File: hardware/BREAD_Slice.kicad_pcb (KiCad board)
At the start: 2 copper layers, 72.6 x 100 mm, 62 parts, among them J1 I2C_01x04, J2 Conn_01x10_Female, J3 Conn_01x02_Socket, J4 Conn_01x02_Socket, J5 Conn_01x02_Socket, J6 Conn_01x02_Socket, Q1 PSMN1R0-30YLC,115, Q2 PSMN1R0-30YLC,115, Q3 PSMN1R0-30YLC,115, Q4 PSMN1R0-30YLC,115, Q5 PSMN1R0-30YLC,115, Q6 PSMN1R0-30YLC,115, Q7 PSMN1R0-30YLC,115, Q8 PSMN1R0-30YLC,115

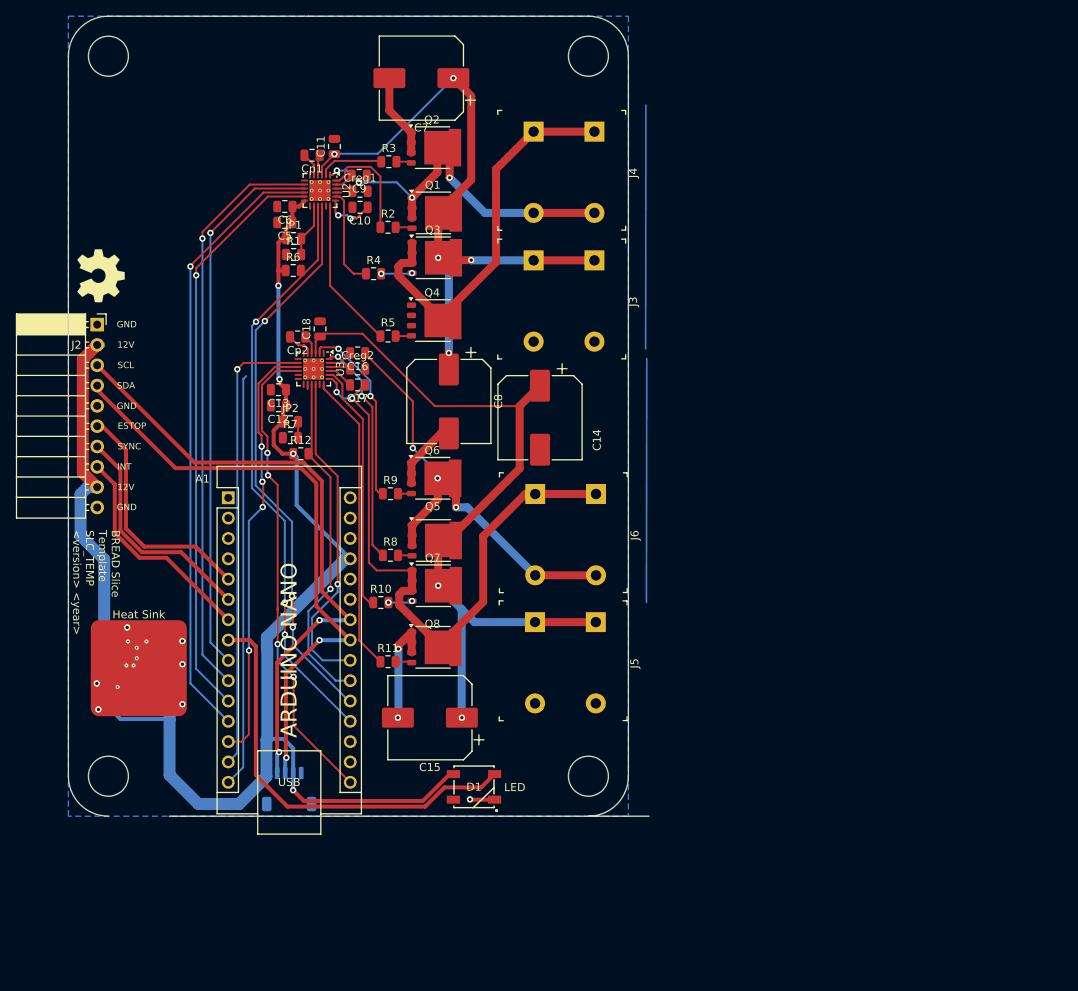
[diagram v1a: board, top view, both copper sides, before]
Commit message: removed old
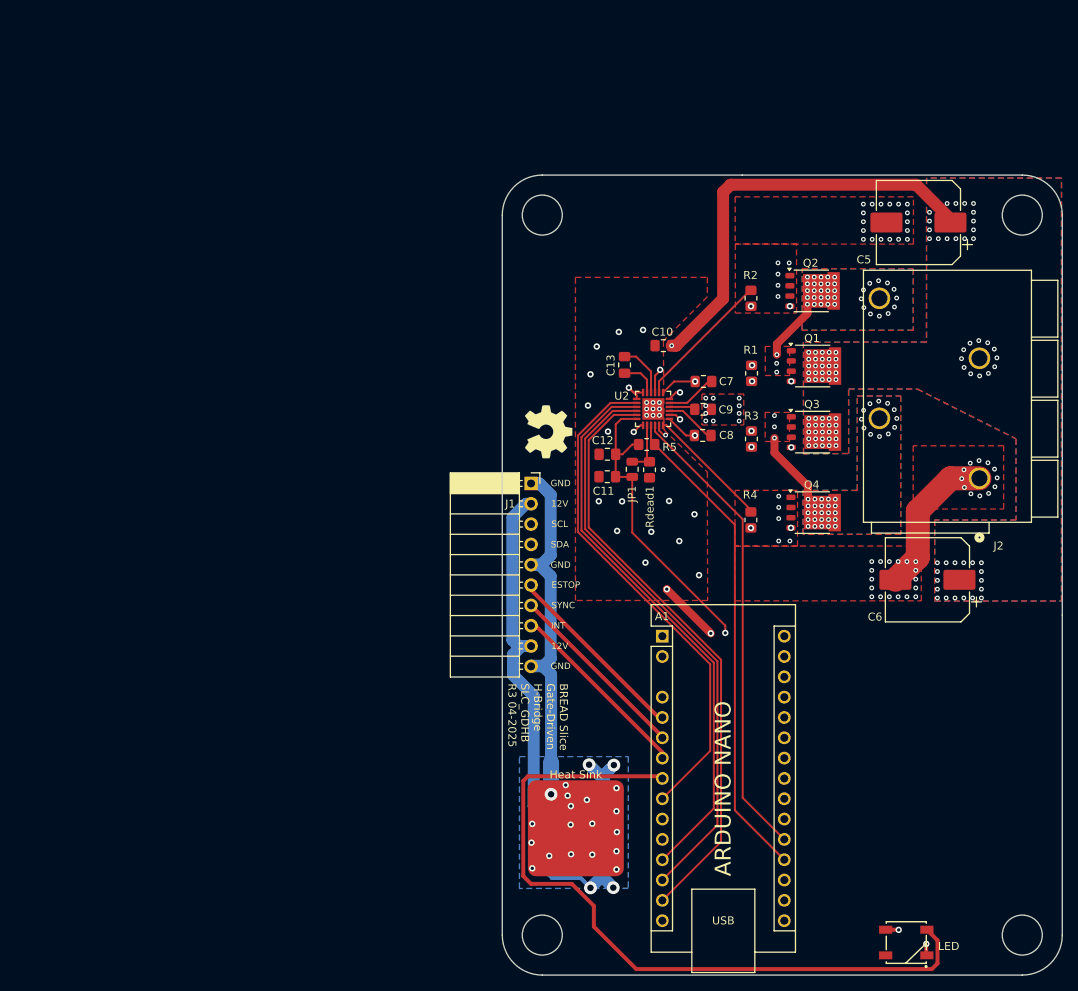
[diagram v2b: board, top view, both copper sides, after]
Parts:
- removed C14, C15: 50V 220uF, Capacitor_SMD:CP_Elec_10x10
- removed C16, C17: 1nF, Capacitor_SMD:C_0805_2012Metric
- removed C18: 50V 10uF, Capacitor_SMD:C_0805_2012Metric
- removed Cp1, Cp2: 16V 470nF, Capacitor_SMD:C_0805_2012Metric
- removed Creg1, Creg2: 16V 22uF, Capacitor_SMD:C_0805_2012Metric
- removed the J1 at (90.8, 121.6)
- removed J3, J4, J5, J6: Conn_01x02_Socket, Library:Term_Block_1x2_P10.16mm
- removed JP2: Jumper_2_Open, Capacitor_SMD:C_0805_2012Metric
- removed Q5, Q6, Q7, Q8: PSMN1R0-30YLC,115, Package_TO_SOT_SMD:LFPAK56
- removed R10, R11, R8, R9: 1K, Capacitor_SMD:C_0805_2012Metric
- removed R12, R6, R7: 10K, Capacitor_SMD:C_0805_2012Metric
- removed U3: ~, Package_DFN_QFN:HVQFN-24-1EP_4x4mm_P0.5mm_EP2.6x2.6mm_ThermalVias
- added J2: 2606-1104/010-000, kml-custom:CONN4_2606-1104&slash_010-000_WAG, F.Cu at (177.1, 82.8)
- added NT1: NetTie_2, NetTie:NetTie-2_SMD_Pad2.0mm, B.Cu at (123.6, 120.3)
- added Rdead1: 3k, Resistor_SMD:R_0805_2012Metric_Pad1.20x1.40mm_HandSolder, F.Cu at (135.9, 81.7)
- C1, C2, C3, C4: footprint Capacitor_SMD:C_1206_3216Metric -> Capacitor_SMD:C_1206_3216Metric_Pad1.33x1.80mm_HandSolder
- C10: value 1nF -> 50V 10uF; footprint Capacitor_SMD:C_0805_2012Metric -> Capacitor_SMD:C_0805_2012Metric_Pad1.18x1.45mm_HandSolder
- C11: value 50V 10uF -> 100nF; footprint Capacitor_SMD:C_0805_2012Metric -> Capacitor_SMD:C_0805_2012Metric_Pad1.18x1.45mm_HandSolder
- C12: footprint Capacitor_SMD:C_0805_2012Metric -> Capacitor_SMD:C_0805_2012Metric_Pad1.18x1.45mm_HandSolder
- C13: value 100nF -> 16V 470nF; footprint Capacitor_SMD:C_0805_2012Metric -> Capacitor_SMD:C_0805_2012Metric_Pad1.18x1.45mm_HandSolder
- C5: value 10uF -> 50V 220uF; footprint Capacitor_SMD:C_0805_2012Metric -> Capacitor_SMD:CP_Elec_10x10
- C6: value 100nF -> 50V 220uF; footprint Capacitor_SMD:C_0805_2012Metric -> Capacitor_SMD:CP_Elec_10x10
- C7, C8: value 50V 220uF -> 1nF; footprint Capacitor_SMD:CP_Elec_10x10 -> Capacitor_SMD:C_0805_2012Metric_Pad1.18x1.45mm_HandSolder
- C9: value 1nF -> 16V 22uF; footprint Capacitor_SMD:C_0805_2012Metric -> Capacitor_SMD:C_0805_2012Metric_Pad1.18x1.45mm_HandSolder
- HS1: footprint KML-Custom:Thermal Pad -> kml-custom:Thermal Pad
- R1: value 10K -> 1K; footprint Capacitor_SMD:C_0805_2012Metric -> Resistor_SMD:R_0805_2012Metric_Pad1.20x1.40mm_HandSolder
- R2, R3, R4: footprint Capacitor_SMD:C_0805_2012Metric -> Resistor_SMD:R_0805_2012Metric_Pad1.20x1.40mm_HandSolder
- R5: value 1K -> 10K; footprint Capacitor_SMD:C_0805_2012Metric -> Resistor_SMD:R_0805_2012Metric_Pad1.20x1.40mm_HandSolder
- U1: value ~ -> AP63205
- U2: value ~ -> A4957SESTR-T; footprint Package_DFN_QFN:HVQFN-24-1EP_4x4mm_P0.5mm_EP2.6x2.6mm_ThermalVias -> kml-custom:QFN-24_ALM
- moved C6 92.9 mm to (170.6, 95.5)
- moved C5 79.2 mm to (169.5, 50.8)
- moved Logo1 59.3 mm to (123.3, 77.0)
- moved R1 59.1 mm to (148.6, 69.7), turned to -90 degrees
- moved HS1 58.2 mm to (126.7, 126.5)
- moved C1 58.0 mm to (123.7, 124.6)
- moved C2 57.8 mm to (126.0, 131.3)
- moved H1 57.8 mm to (122.5, 49.9)
- moved H2 57.8 mm to (122.5, 139.9)
- moved J1 57.8 mm to (121.1, 83.4)
- moved U1 57.8 mm to (123.6, 127.8)
- moved C3 57.8 mm to (128.7, 124.5)
- moved H3 57.8 mm to (182.5, 49.9)
- moved H4 57.8 mm to (182.5, 139.9)
- moved L1 57.8 mm to (128.7, 127.8)
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- renumbered J2 to J1
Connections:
- net /E_STOP renamed /ESTOP
- A1 pad 10: /BLO1 -> unconnected-(A1-D7-Pad10)
- A1 pad 11: /AHI1 -> unconnected-(A1-D8-Pad11)
- A1 pad 12: /ALO1 -> /BHI1
- A1 pad 13: /BHI2 -> /ALO1
- A1 pad 14: /BLO2 -> /ALI1
- A1 pad 15: /AHI2 -> unconnected-(A1-D12-Pad15)
- A1 pad 16: /ALO2 -> unconnected-(A1-D13-Pad16)
- A1 pad 21: /FAULT2 -> unconnected-(A1-A2-Pad21)
- A1 pad 22: /RESET2 -> unconnected-(A1-A3-Pad22)
- A1 pad 9: /BHI1 -> /BLO1
- C10 pad 1: /A4947 H-Bridge/SB -> /VBB1
- C10 pad 2: Net-(U2-CB) -> GND
- C11 pad 1: /A4947 H-Bridge/VBB -> +5V
- C13 pad 1: +5V -> Net-(U2-CP1)
- C13 pad 2: GND -> Net-(U2-CP2)
- C5 pad 1: +5V -> /VBB1
- C6 pad 1: +5V -> /VBB1
- C7 pad 1: /A4947 H-Bridge/VBB -> /A4947 H-Bridge/SA
- C7 pad 2: GND -> /A4947 H-Bridge/CA
- C8 pad 1: /A4947 H-Bridge/VBB -> /A4947 H-Bridge/SB
- C8 pad 2: GND -> /A4947 H-Bridge/CB
- C9 pad 1: /A4947 H-Bridge/SA -> /A4947 H-Bridge/VREG
- C9 pad 2: Net-(U2-CA) -> GND
- J1 pad 1: GND -> GNDPWR
- J1 pad 10: GND -> GNDPWR
- J1 pad 5: GND -> GNDPWR
- Q1 pad 5: /A4947 H-Bridge/VBB -> /VBB1
- Q3 pad 5: /A4947 H-Bridge/VBB -> /VBB1
- R1 pad 1: GND -> /A4947 H-Bridge/GHA
- R1 pad 2: /A4947 H-Bridge/RDEAD -> Net-(Q1-G)
- R2 pad 1: /A4947 H-Bridge/GHA -> /A4947 H-Bridge/GLA
- R2 pad 2: Net-(Q1-G) -> Net-(Q2-G)
- R3 pad 1: /A4947 H-Bridge/GLA -> /A4947 H-Bridge/GHB
- R3 pad 2: Net-(Q2-G) -> Net-(Q3-G)
- R4 pad 1: /A4947 H-Bridge/GHB -> /A4947 H-Bridge/GLB
- R4 pad 2: Net-(Q3-G) -> Net-(Q4-G)
- R5 pad 1: /A4947 H-Bridge/GLB -> +5V
- R5 pad 2: Net-(Q4-G) -> /FAULT1
- U2 pad 11: /AHI1 -> /ALI1
- U2 pad 21: Net-(U2-CB) -> /A4947 H-Bridge/CB
- U2 pad 22: Net-(U2-VREG) -> /A4947 H-Bridge/VREG
- U2 pad 23: Net-(U2-CA) -> /A4947 H-Bridge/CA
- U2 pad 25: unconnected-(U2-PAD-Pad25)_6 -> GND
- U2 pad 3: /A4947 H-Bridge/VBB -> /VBB1
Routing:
- net /A4947 H-Bridge1/VBB: track 97.3 -> 0.00 mm, vias 2 -> 0
- net +5V: track 160.6 -> 72.3 mm, vias 4 -> 6
- net /A4947 H-Bridge/VBB: track 81.3 -> 0.00 mm, vias 5 -> 0
- net /A4947 H-Bridge1/SB: track 79.6 -> 0.00 mm, vias 2 -> 0
- net /ALI1: track 0.00 -> 74.7 mm
- net /AHI1: track 73.0 -> 0.00 mm, vias 1 -> 0
- net /VBB1: track 0.00 -> 59.9 mm, vias 0 -> 98
- net /ALO2: track 59.7 -> 0.00 mm, vias 4 -> 0
- net /BLO2: track 57.5 -> 0.00 mm, vias 1 -> 0
- net /A4947 H-Bridge1/SA: track 54.8 -> 0.00 mm, vias 3 -> 0
- net /BHI2: track 53.6 -> 0.00 mm, vias 4 -> 0
- net /AHI2: track 51.9 -> 0.00 mm
- net GNDPWR: track 0.00 -> 43.7 mm
- net /FAULT2: track 42.8 -> 0.00 mm, vias 1 -> 0
- net /RESET2: track 41.0 -> 0.00 mm, vias 1 -> 0
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- added copper zone on In1.Cu, net +5V
- added copper zone on B.Cu, net /A4947 H-Bridge/SA
- added copper zone on F.Cu, net /A4947 H-Bridge/SA
- added copper zone on B.Cu, net /A4947 H-Bridge/SB
- added copper zone on F.Cu, net /A4947 H-Bridge/SB
- added copper zone on B.Cu, net /VBB1
- added copper zone on F.Cu, net /VBB1
- added copper zone on F.Cu, net GND
- added copper zone on In2.Cu, net GND
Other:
- board size 72.6 x 100 mm -> 70 x 100 mm
- copper layers 2 -> 4
- board text added: "BREAD Slice Gate-Driven H-Bridge SLC_GDHB R3 04-2025"
- board text added: "L1 (Top): - All FETs and high-current copper pours (VBB, SA, SB) - Primary routing for motor power and gate drive signals - Thick copper (2-3 oz) - Thermal via arrays under FETs and A4957 exposed pad - Minimal digital traces; avoid signal routing near power zones L2 (Inner 1): - Signal layer for logic routing L3 (Inner 2): - Solid ground plane (1-2 oz) - Connect all IC grounds, FET sources, and t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"
- board text added: "L1 (Top): - Routing L2 (Inner 1): - 5V L3 (Inner 2): - GND L4 (Bottom): - 12-->5V regulator"
- board text added: "MOTOR+"
- board text added: "MOTOR-"
- board text added: "PWR GND"
- board text added: "PWR IN"
- board text removed: "5V I2C Connector"
- board text removed: "BREAD Slice Template SLC_TEMP <version> <year>"
